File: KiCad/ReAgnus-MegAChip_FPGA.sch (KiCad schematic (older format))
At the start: 5 parts, among them J2 Conn_02x05_Odd_Even, U10 AS4C4M16SA, U7 GW1N-UV9LQ144

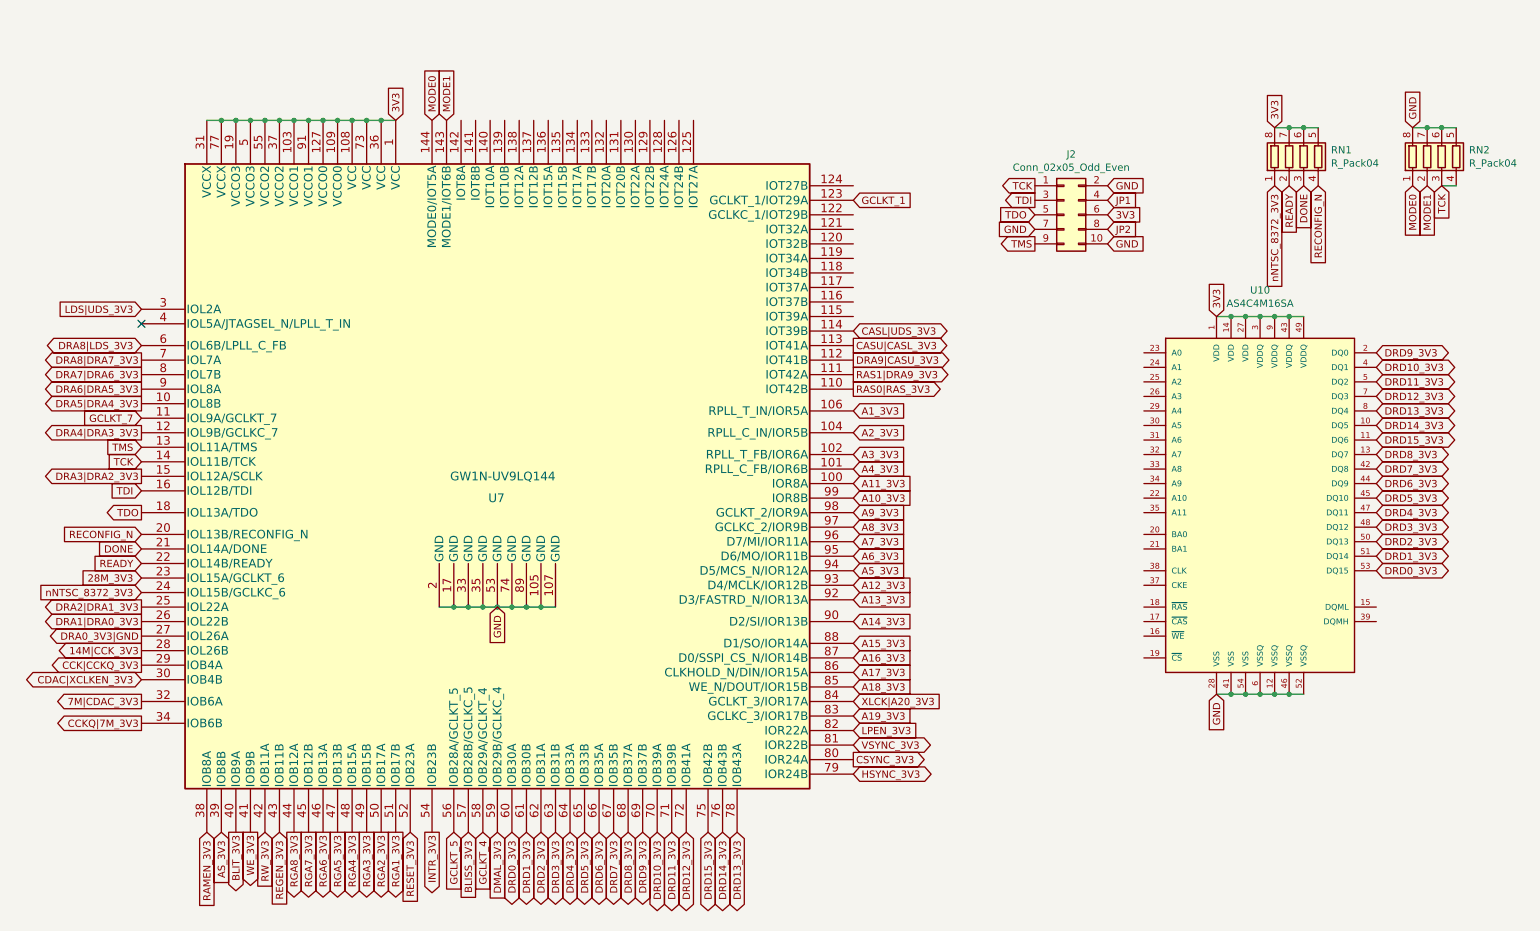
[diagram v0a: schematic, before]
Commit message: more routing
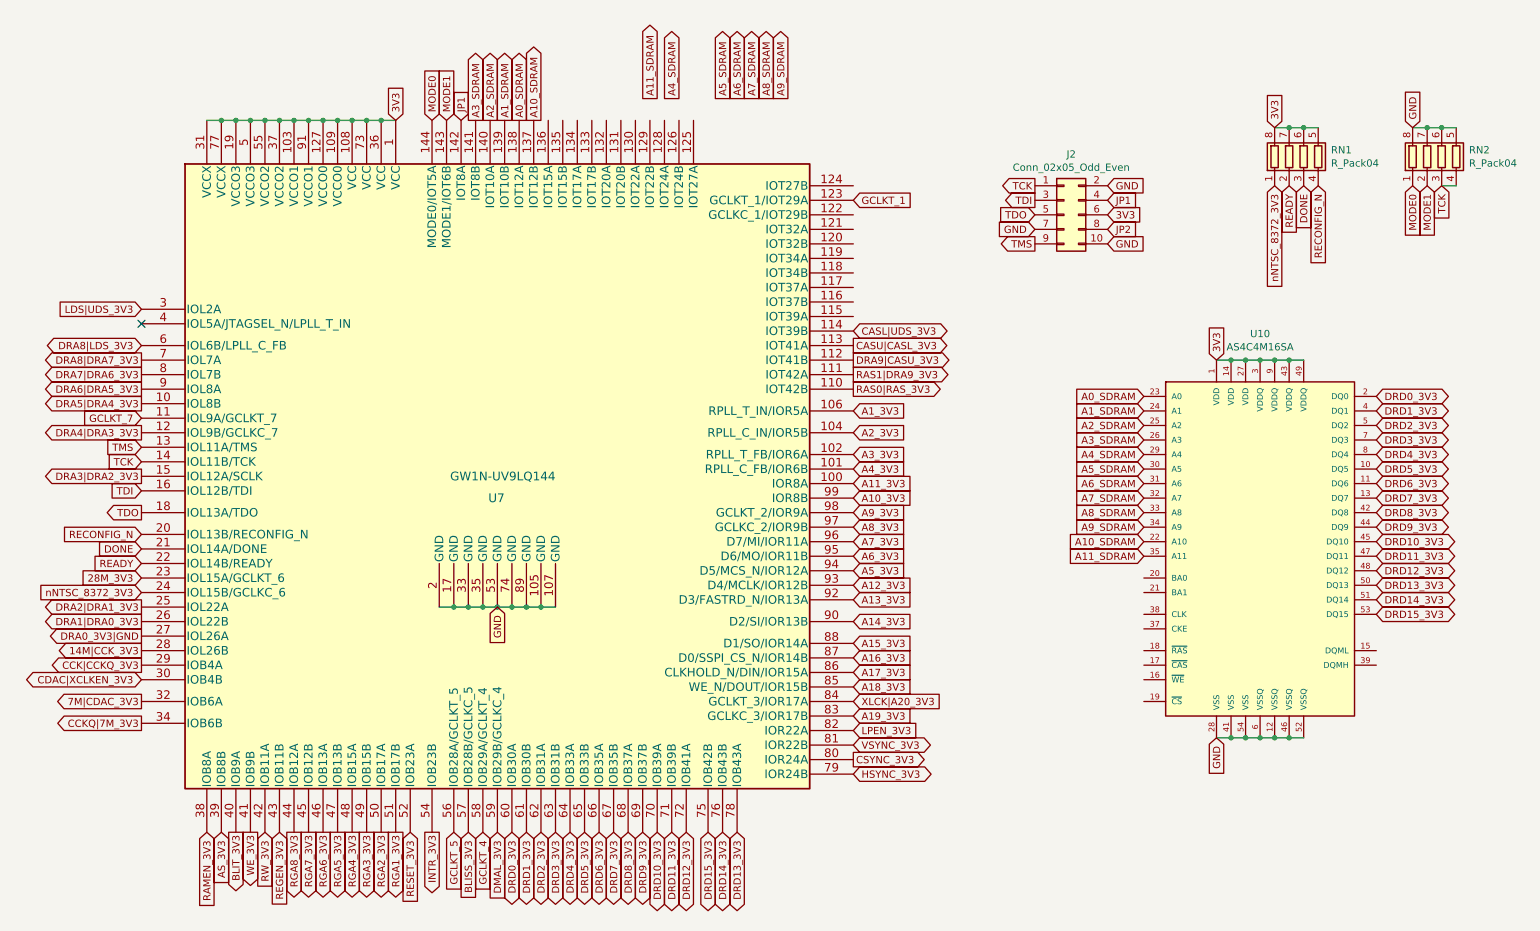
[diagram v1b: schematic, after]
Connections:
- net DRD0_3V3: now also U10.2 (DQ0); no longer U10.53 (DQ15)
- net DRD10_3V3: now also U10.45 (DQ10); no longer U10.4 (DQ1)
- net DRD11_3V3: now also U10.47 (DQ11); no longer U10.5 (DQ2)
- net DRD12_3V3: now also U10.48 (DQ12); no longer U10.7 (DQ3)
- net DRD13_3V3: now also U10.50 (DQ13); no longer U10.8 (DQ4)
- net DRD14_3V3: now also U10.51 (DQ14); no longer U10.10 (DQ5)
- net DRD15_3V3: now also U10.53 (DQ15); no longer U10.11 (DQ6)
- net DRD1_3V3: now also U10.4 (DQ1); no longer U10.51 (DQ14)
- net DRD2_3V3: now also U10.5 (DQ2); no longer U10.50 (DQ13)
- net DRD3_3V3: now also U10.7 (DQ3); no longer U10.48 (DQ12)
- net DRD4_3V3: now also U10.8 (DQ4); no longer U10.47 (DQ11)
- net DRD5_3V3: now also U10.10 (DQ5); no longer U10.45 (DQ10)
- net DRD6_3V3: now also U10.11 (DQ6); no longer U10.44 (DQ9)
- net DRD7_3V3: now also U10.13 (DQ7); no longer U10.42 (DQ8)
- net DRD8_3V3: now also U10.42 (DQ8); no longer U10.13 (DQ7)
- net DRD9_3V3: now also U10.44 (DQ9); no longer U10.2 (DQ0)
- net JP1: now also U7.142 (IOT8A)
- net A10_SDRAM: now reaches U10.22 (A10)
- net A10_SDRAM: now also U7.137 (IOT12B)
- net A0_SDRAM: now reaches U10.23 (A0)
- net A0_SDRAM: now also U7.138 (IOT12A)
- net A1_SDRAM: now reaches U10.24 (A1)
- net A1_SDRAM: now also U7.139 (IOT10B)
- net A2_SDRAM: now reaches U10.25 (A2)
- net A2_SDRAM: now also U7.140 (IOT10A)
- net A3_SDRAM: now reaches U10.26 (A3)
- net A3_SDRAM: now also U7.141 (IOT8B)
- net A4_SDRAM: now reaches U10.29 (A4)
- net A5_SDRAM: now reaches U10.30 (A5)
- net A6_SDRAM: now reaches U10.31 (A6)
- net A7_SDRAM: now reaches U10.32 (A7)
- net A8_SDRAM: now reaches U10.33 (A8)
- net A9_SDRAM: now reaches U10.34 (A9)
- net A11_SDRAM: now reaches U10.35 (A11)
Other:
- moved on the sheet: U10
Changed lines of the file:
@@
 L Memory_RAM:AS4C4M16SA U10
 U 1 1 632B4228
-P 9150 3700
-F 0 "U10" H 9150 5181 50  0000 C CNN
-F 1 "AS4C4M16SA" H 9150 5090 50  0000 C CNN
-F 2 "Package_SO:TSOP-II-54_22.2x10.16mm_P0.8mm" H 9150 3700 50  0001 C CIN
-F 3 "https://www.alliancememory.com/wp-content/uploads/pdf/dram/64M-AS4C4M16SA-CI_v3.0_March%202015.pdf" H 9150 3450 50  0001 C CNN
-	1    9150 3700
+P 9150 4000
+F 0 "U10" H 9150 5481 50  0000 C CNN
+F 1 "AS4C4M16SA" H 9150 5390 50  0000 C CNN
+F 2 "Package_SO:TSOP-II-54_22.2x10.16mm_P0.8mm" H 9150 4000 50  0001 C CIN
+F 3 "https://www.alliancememory.com/wp-content/uploads/pdf/dram/64M-AS4C4M16SA-CI_v3.0_March%202015.pdf" H 9150 3750 50  0001 C CNN
+	1    9150 4000
 	1    0    0    -1
 $EndComp
-Text GLabel 9950 4150 2    50   BiDi ~ 0
+Text GLabel 9950 2950 2    50   BiDi ~ 0
 DRD0_3V3
-Text GLabel 9950 4050 2    50   BiDi ~ 0
+Text GLabel 9950 3050 2    50   BiDi ~ 0
 DRD1_3V3
-Text GLabel 9950 3950 2    50   BiDi ~ 0
+Text GLabel 9950 3150 2    50   BiDi ~ 0
 DRD2_3V3
-Text GLabel 9950 3850 2    50   BiDi ~ 0
+Text GLabel 9950 3250 2    50   BiDi ~ 0
 DRD3_3V3
-Text GLabel 9950 3750 2    50   BiDi ~ 0
+Text GLabel 9950 3350 2    50   BiDi ~ 0
 DRD4_3V3
-Text GLabel 9950 3650 2    50   BiDi ~ 0
+Text GLabel 9950 3450 2    50   BiDi ~ 0
 DRD5_3V3
 Text GLabel 9950 3550 2    50   BiDi ~ 0
 DRD6_3V3
-Text GLabel 9950 3450 2    50   BiDi ~ 0
+Text GLabel 9950 3650 2    50   BiDi ~ 0
 DRD7_3V3
-Text GLabel 9950 3350 2    50   BiDi ~ 0
+Text GLabel 9950 3750 2    50   BiDi ~ 0
 DRD8_3V3
-Text GLabel 9950 2650 2    50   BiDi ~ 0
+Text GLabel 9950 3850 2    50   BiDi ~ 0
 DRD9_3V3
-Text GLabel 9950 2750 2    50   BiDi ~ 0
+Text GLabel 9950 3950 2    50   BiDi ~ 0
 DRD10_3V3
-Text GLabel 9950 2850 2    50   BiDi ~ 0
+Text GLabel 9950 4050 2    50   BiDi ~ 0
 DRD11_3V3
-Text GLabel 9950 2950 2    50   BiDi ~ 0
+Text GLabel 9950 4150 2    50   BiDi ~ 0
 DRD12_3V3
-Text GLabel 9950 3050 2    50   BiDi ~ 0
+Text GLabel 9950 4250 2    50   BiDi ~ 0
 DRD13_3V3
-Text GLabel 9950 3150 2    50   BiDi ~ 0
+Text GLabel 9950 4350 2    50   BiDi ~ 0
 DRD14_3V3
-Text GLabel 9950 3250 2    50   BiDi ~ 0
+Text GLabel 9950 4450 2    50   BiDi ~ 0
 DRD15_3V3
-Text GLabel 8850 2400 1    50   Input ~ 0
+Text GLabel 8850 2700 1    50   Input ~ 0
 3V3
 Wire Wire Line
-	8850 2400 8950 2400
-Connection ~ 8950 2400
+	8850 2700 8950 2700
+Connection ~ 8950 2700
 Wire Wire Line
-	8950 2400 9050 2400
-Connection ~ 9050 2400
+	8950 2700 9050 2700
+Connection ~ 9050 2700
 Wire Wire Line
-	9050 2400 9150 2400
-Connection ~ 9150 2400
+	9050 2700 9150 2700
+Connection ~ 9150 2700
 Wire Wire Line
-	9150 2400 9250 2400
-Connection ~ 9250 2400
+	9150 2700 9250 2700
+Connection ~ 9250 2700
 Wire Wire Line
-	9250 2400 9350 2400
-Connection ~ 9350 2400
+	9250 2700 9350 2700
+Connection ~ 9350 2700
 Wire Wire Line
-	9350 2400 9450 2400
-Text GLabel 8850 5000 3    50   Input ~ 0
+	9350 2700 9450 2700
+Text GLabel 8850 5300 3    50   Input ~ 0
 GND
 Wire Wire Line
-	8850 5000 8950 5000
-Connection ~ 8950 5000
+	8850 5300 8950 5300
+Connection ~ 8950 5300
 Wire Wire Line
-	8950 5000 9050 5000
-Connection ~ 9050 5000
+	8950 5300 9050 5300
+Connection ~ 9050 5300
 Wire Wire Line
-	9050 5000 9150 5000
-Connection ~ 9150 5000
+	9050 5300 9150 5300
+Connection ~ 9150 5300
 Wire Wire Line
-	9150 5000 9250 5000
-Connection ~ 9250 5000
+	9150 5300 9250 5300
+Connection ~ 9250 5300
 Wire Wire Line
-	9250 5000 9350 5000
-Connection ~ 9350 5000
+	9250 5300 9350 5300
+Connection ~ 9350 5300
 Wire Wire Line
-	9350 5000 9450 5000
+	9350 5300 9450 5300
 Text GLabel 1450 4300 0    50   Input ~ 0
 nNTSC_8372_3V3
@@
 Wire Wire Line
 	10400 1500 10500 1500
+Text GLabel 8350 2950 0    50   Input ~ 0
+A0_SDRAM
+Text GLabel 8350 3050 0    50   Input ~ 0
+A1_SDRAM
+Text GLabel 8350 3150 0    50   Input ~ 0
+A2_SDRAM
+Text GLabel 8350 3250 0    50   Input ~ 0
+A3_SDRAM
+Text GLabel 8350 3350 0    50   Input ~ 0
+A4_SDRAM
+Text GLabel 8350 3450 0    50   Input ~ 0
+A5_SDRAM
+Text GLabel 8350 3550 0    50   Input ~ 0
+A6_SDRAM
+Text GLabel 8350 3650 0    50   Input ~ 0
+A7_SDRAM
+Text GLabel 8350 3750 0    50   Input ~ 0
+A8_SDRAM
+Text GLabel 8350 3850 0    50   Input ~ 0
+A9_SDRAM
+Text GLabel 8350 3950 0    50   Input ~ 0
+A10_SDRAM
+Text GLabel 8350 4050 0    50   Input ~ 0
+A11_SDRAM
+Text GLabel 4050 1050 1    50   Output ~ 0
+A0_SDRAM
+Text GLabel 3950 1050 1    50   Output ~ 0
+A1_SDRAM
+Text GLabel 3850 1050 1    50   Output ~ 0
+A2_SDRAM
+Text GLabel 3750 1050 1    50   Output ~ 0
+A3_SDRAM
+Text GLabel 5100 900  1    50   Output ~ 0
+A4_SDRAM
+Text GLabel 5450 900  1    50   Output ~ 0
+A5_SDRAM
+Text GLabel 5550 900  1    50   Output ~ 0
+A6_SDRAM
+Text GLabel 5650 900  1    50   Output ~ 0
+A7_SDRAM
+Text GLabel 5750 900  1    50   Output ~ 0
+A8_SDRAM
+Text GLabel 5850 900  1    50   Output ~ 0
+A9_SDRAM
+Text GLabel 4150 1050 1    50   Output ~ 0
+A10_SDRAM
+Text GLabel 4950 900  1    50   Output ~ 0
+A11_SDRAM
+Text GLabel 3650 1050 1    50   Input ~ 0
+JP1
 $EndSCHEMATC

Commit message: more routing
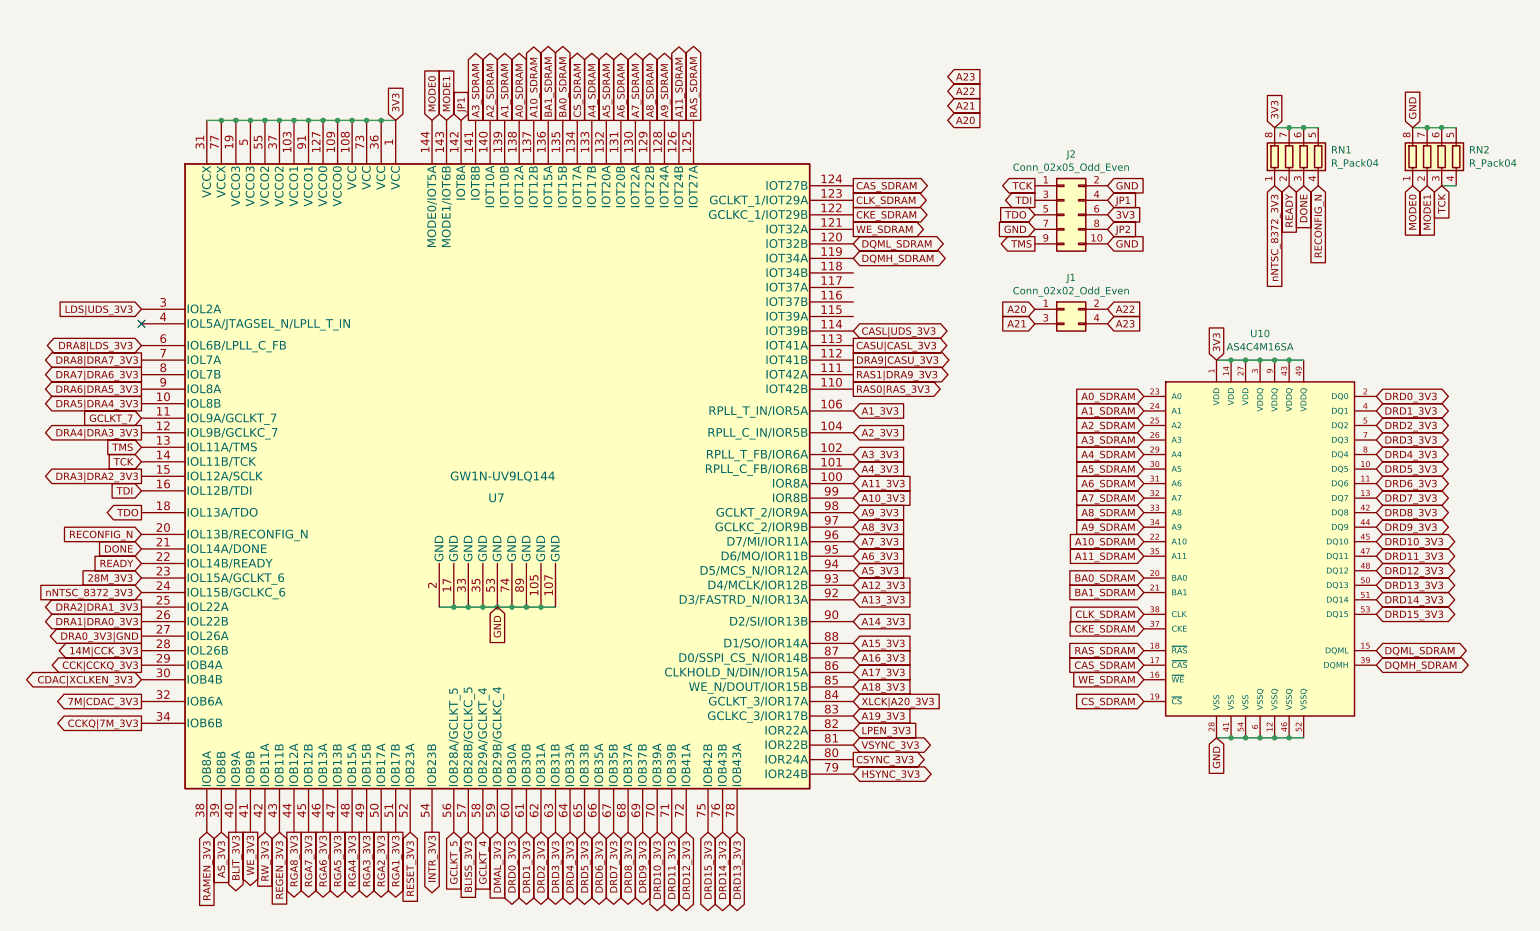
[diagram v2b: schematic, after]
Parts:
- added J1: Conn_02x02_Odd_Even, Connector_PinHeader_2.00mm:PinHeader_2x02_P2.00mm_Vertical, symbol Connector_Generic:Conn_02x02_Odd_Even
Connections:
- net GCLKT_1 is gone; now on net CLK_SDRAM: U7.123 (GCLKT_1/IOT29A)
- net A11_SDRAM: now also U7.126 (IOT24B)
- net A4_SDRAM: now also U7.133 (IOT17B)
- net A5_SDRAM: now also U7.132 (IOT20A)
- net A6_SDRAM: now also U7.131 (IOT20B)
- net A7_SDRAM: now also U7.130 (IOT22A)
- net A8_SDRAM: now also U7.129 (IOT22B)
- net A9_SDRAM: now also U7.128 (IOT24A)
- net DQML_SDRAM: now reaches U10.15 (DQML)
- net DQML_SDRAM: now also U7.120 (IOT32B)
- net WE_SDRAM: now reaches U10.16 (~WE~)
- net WE_SDRAM: now also U7.121 (IOT32A)
- net CAS_SDRAM: now reaches U10.17 (~CAS~)
- net CAS_SDRAM: now also U7.124 (IOT27B)
- net RAS_SDRAM: now reaches U10.18 (~RAS~)
- net RAS_SDRAM: now also U7.125 (IOT27A)
- net CS_SDRAM: now reaches U10.19 (~CS~)
- net CS_SDRAM: now also U7.134 (IOT17A)
- net BA0_SDRAM: now reaches U10.20 (BA0)
- net BA0_SDRAM: now also U7.135 (IOT15B)
- net BA1_SDRAM: now reaches U10.21 (BA1)
- net BA1_SDRAM: now also U7.136 (IOT15A)
- net CKE_SDRAM: now reaches U10.37 (CKE)
- net CKE_SDRAM: now also U7.122 (GCLKC_1/IOT29B)
- net CLK_SDRAM: now reaches U10.38 (CLK)
- net DQMH_SDRAM: now reaches U10.39 (DQMH)
- net DQMH_SDRAM: now also U7.119 (IOT34A)
- new net A20: J1.1 (Pin_1)
- new net A21: J1.3 (Pin_3)
- new net A22: J1.2 (Pin_2)
- new net A23: J1.4 (Pin_4)
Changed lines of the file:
@@
 Text GLabel 3800 5950 3    50   Input ~ 0
 GCLKT_4
-Text GLabel 6350 1600 2    50   Input ~ 0
-GCLKT_1
 Text GLabel 3550 1050 1    50   Input ~ 0
 MODE1
@@
 Text GLabel 3750 1050 1    50   Output ~ 0
 A3_SDRAM
-Text GLabel 5100 900  1    50   Output ~ 0
+Text GLabel 4550 1050 1    50   Output ~ 0
 A4_SDRAM
-Text GLabel 5450 900  1    50   Output ~ 0
+Text GLabel 4650 1050 1    50   Output ~ 0
 A5_SDRAM
-Text GLabel 5550 900  1    50   Output ~ 0
+Text GLabel 4750 1050 1    50   Output ~ 0
 A6_SDRAM
-Text GLabel 5650 900  1    50   Output ~ 0
+Text GLabel 4850 1050 1    50   Output ~ 0
 A7_SDRAM
-Text GLabel 5750 900  1    50   Output ~ 0
+Text GLabel 4950 1050 1    50   Output ~ 0
 A8_SDRAM
-Text GLabel 5850 900  1    50   Output ~ 0
+Text GLabel 5050 1050 1    50   Output ~ 0
 A9_SDRAM
 Text GLabel 4150 1050 1    50   Output ~ 0
 A10_SDRAM
-Text GLabel 4950 900  1    50   Output ~ 0
+Text GLabel 5150 1050 1    50   Output ~ 0
 A11_SDRAM
 Text GLabel 3650 1050 1    50   Input ~ 0
 JP1
+Text GLabel 8350 4200 0    50   Input ~ 0
+BA0_SDRAM
+Text GLabel 8350 4300 0    50   Input ~ 0
+BA1_SDRAM
+Text GLabel 4350 1050 1    50   Output ~ 0
+BA0_SDRAM
+Text GLabel 4250 1050 1    50   Output ~ 0
+BA1_SDRAM
+Text GLabel 8350 4450 0    50   Input ~ 0
+CLK_SDRAM
+Text GLabel 8350 4550 0    50   Input ~ 0
+CKE_SDRAM
+Text GLabel 8350 5050 0    50   Input ~ 0
+CS_SDRAM
+Text GLabel 8350 4700 0    50   Input ~ 0
+RAS_SDRAM
+Text GLabel 8350 4800 0    50   Input ~ 0
+CAS_SDRAM
+Text GLabel 8350 4900 0    50   Input ~ 0
+WE_SDRAM
+Text GLabel 9950 4700 2    50   BiDi ~ 0
+DQML_SDRAM
+Text GLabel 9950 4800 2    50   BiDi ~ 0
+DQMH_SDRAM
+Text GLabel 4450 1050 1    50   Output ~ 0
+CS_SDRAM
+Text GLabel 5250 1050 1    50   Output ~ 0
+RAS_SDRAM
+Text GLabel 6350 1500 2    50   Output ~ 0
+CAS_SDRAM
+Text GLabel 6350 1800 2    50   Output ~ 0
+WE_SDRAM
+Text GLabel 6350 1900 2    50   BiDi ~ 0
+DQML_SDRAM
+Text GLabel 6350 1600 2    50   Output ~ 0
+CLK_SDRAM
+Text GLabel 6350 1700 2    50   Output ~ 0
+CKE_SDRAM
+Text GLabel 6350 2000 2    50   BiDi ~ 0
+DQMH_SDRAM
+Text GLabel 7000 1050 2    50   Input ~ 0
+A20
+Text GLabel 7000 950  2    50   Input ~ 0
+A21
+Text GLabel 7000 850  2    50   Input ~ 0
+A22
+Text GLabel 7000 750  2    50   Input ~ 0
+A23
+Text GLabel 8100 2350 2    50   Input ~ 0
+A22
+Text GLabel 8100 2450 2    50   Input ~ 0
+A23
+$Comp
+L Connector_Generic:Conn_02x02_Odd_Even J1
+U 1 1 636B90A6
+P 7800 2350
+F 0 "J1" H 7850 2567 50  0000 C CNN
+F 1 "Conn_02x02_Odd_Even" H 7850 2476 50  0000 C CNN
+F 2 "Connector_PinHeader_2.00mm:PinHeader_2x02_P2.00mm_Vertical" H 7800 2350 50  0001 C CNN
+F 3 "~" H 7800 2350 50  0001 C CNN
+	1    7800 2350
+	1    0    0    -1
+$EndComp
+Text GLabel 7600 2450 0    50   Input ~ 0
+A21
+Text GLabel 7600 2350 0    50   Input ~ 0
+A20
 $EndSCHEMATC
